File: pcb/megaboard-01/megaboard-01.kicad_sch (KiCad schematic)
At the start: 31 parts, among them J1 Conn_01x01_Pin, J2 Conn_01x01_Pin, J3 Conn_01x03_Pin, J4 Conn_01x01_Pin, J5 Conn_01x01_Pin, J6 C37208, J7 Conn_01x02_Pin, J8 Conn_01x02_Pin, T1 SWB1040-PCL, U1 THS3091DDAR, U2 AD9833xRM, X1 C558756

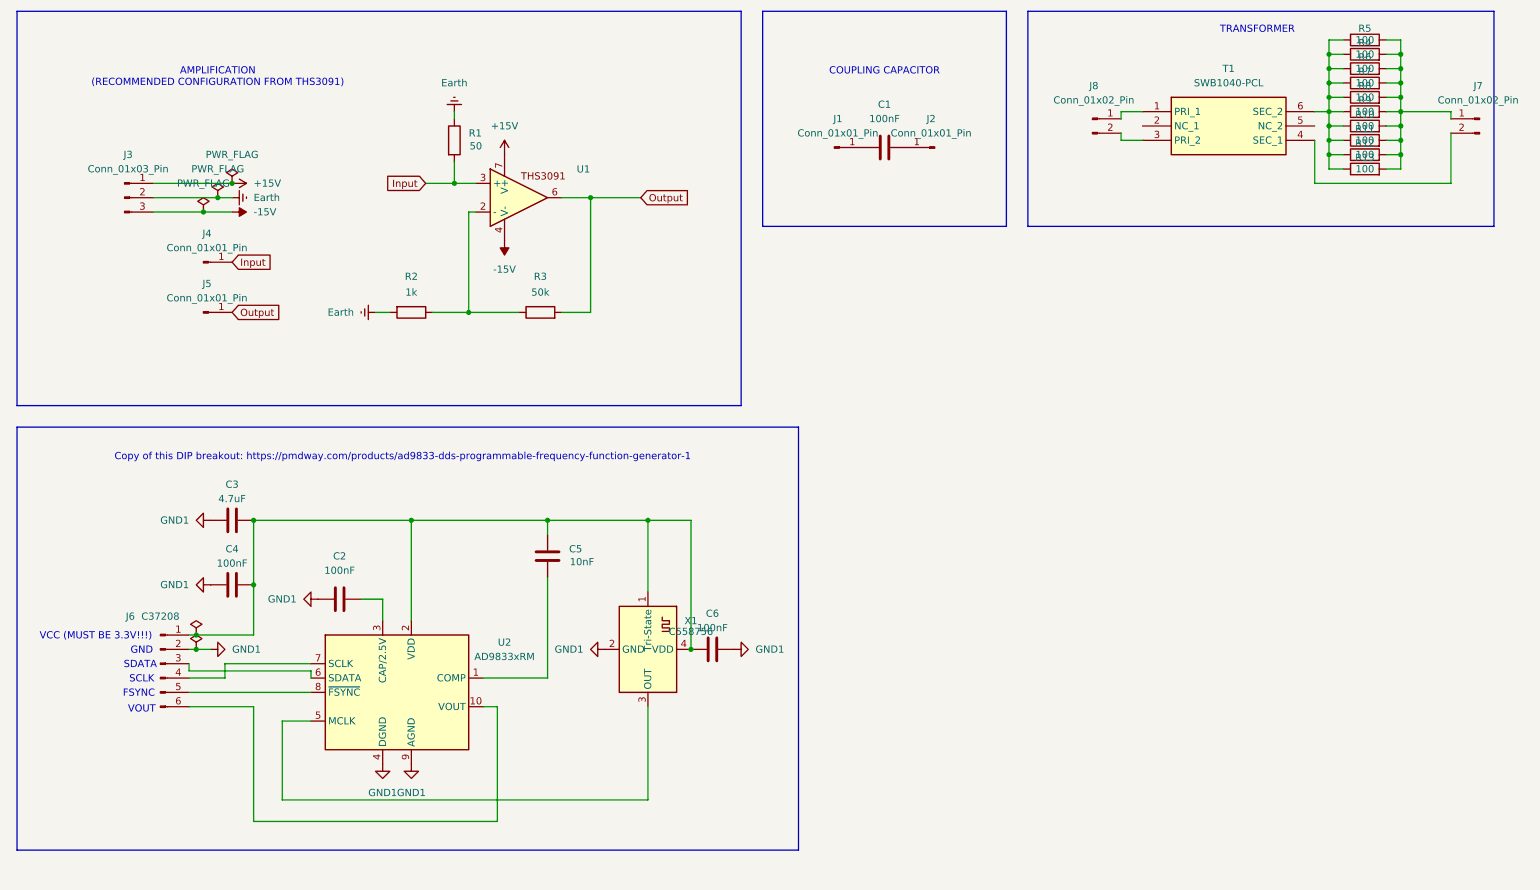
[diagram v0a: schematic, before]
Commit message: stuff
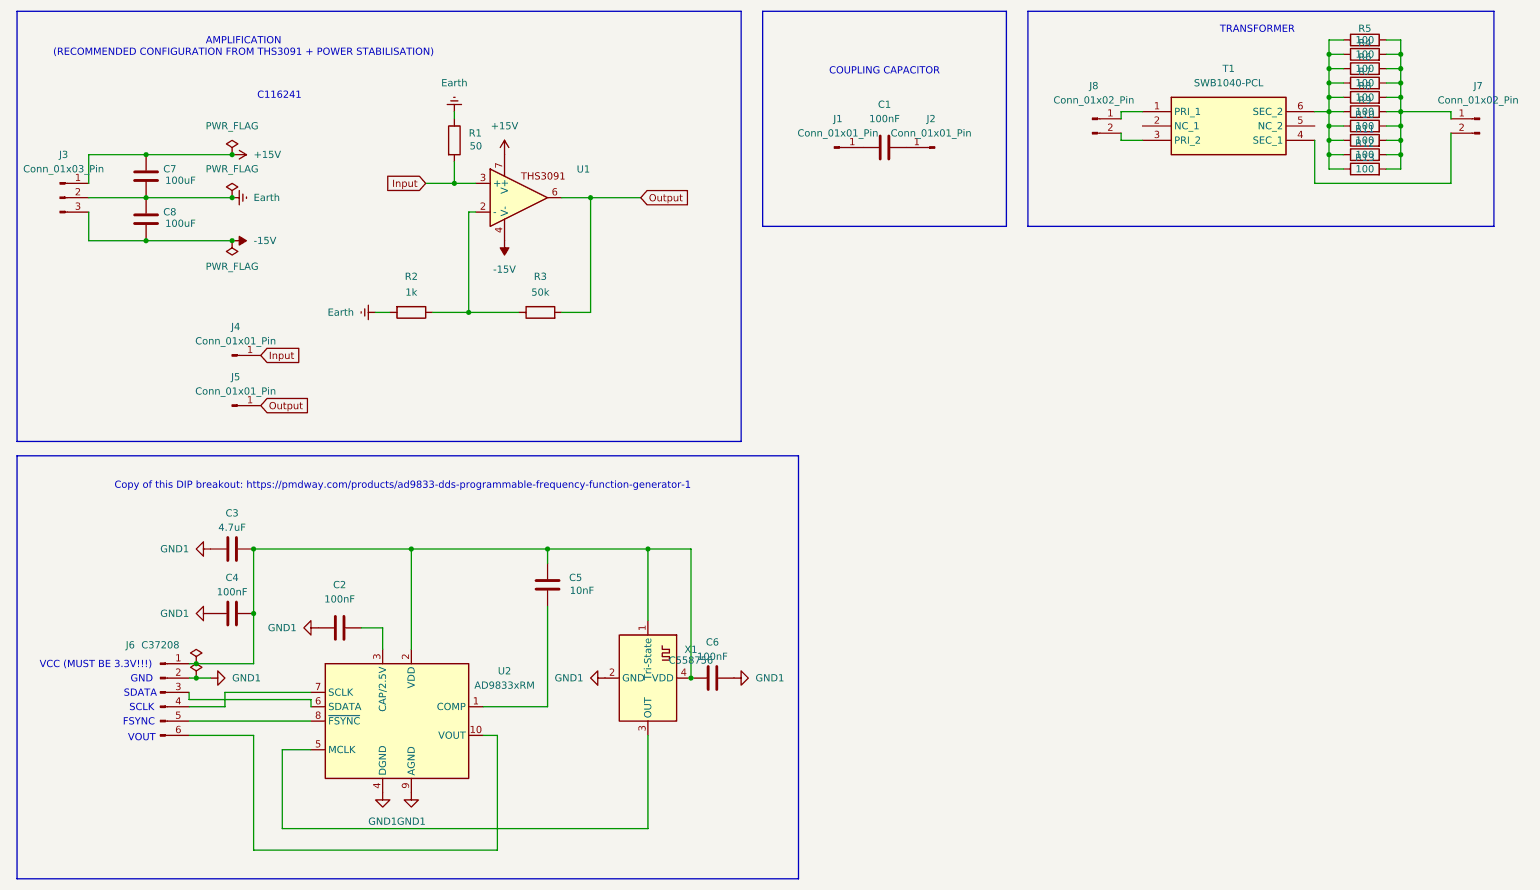
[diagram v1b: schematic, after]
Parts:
- added C7, C8: C116241, Capacitor_SMD:CP_Elec_8x10, symbol Device:C
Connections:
- net +15V: now also C7.1
- net -15V: now also C8.2
- net Earth: now also C7.2, C8.1
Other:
- note added: "AMPLIFICATION (RECOMMENDED CONFIGURATION FROM THS3091 + POWER STABILISATION)"
- note added: "C116241"
- note removed: "AMPLIFICATION (RECOMMENDED CONFIGURATION FROM THS3091)"
- moved on the sheet: C2, C3, C4, C5, C6, J3, J4, J5, J6, U2, X1
